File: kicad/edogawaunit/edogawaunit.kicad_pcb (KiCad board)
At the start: 2 copper layers, 26.7 x 22.9 mm, 11 parts, among them J1 Conn_01x03, J2 Conn_01x02, J3 Conn_01x02, SW1 SW_Push, U1 TLP222A-2

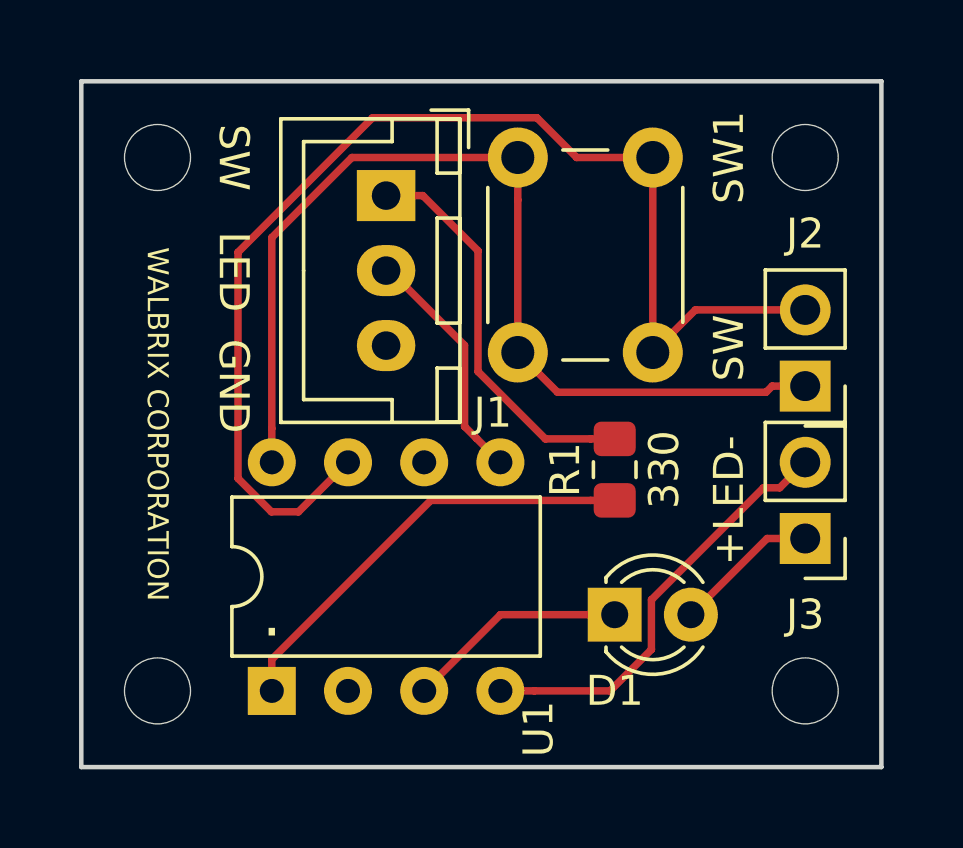
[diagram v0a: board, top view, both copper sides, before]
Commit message: PCBs update
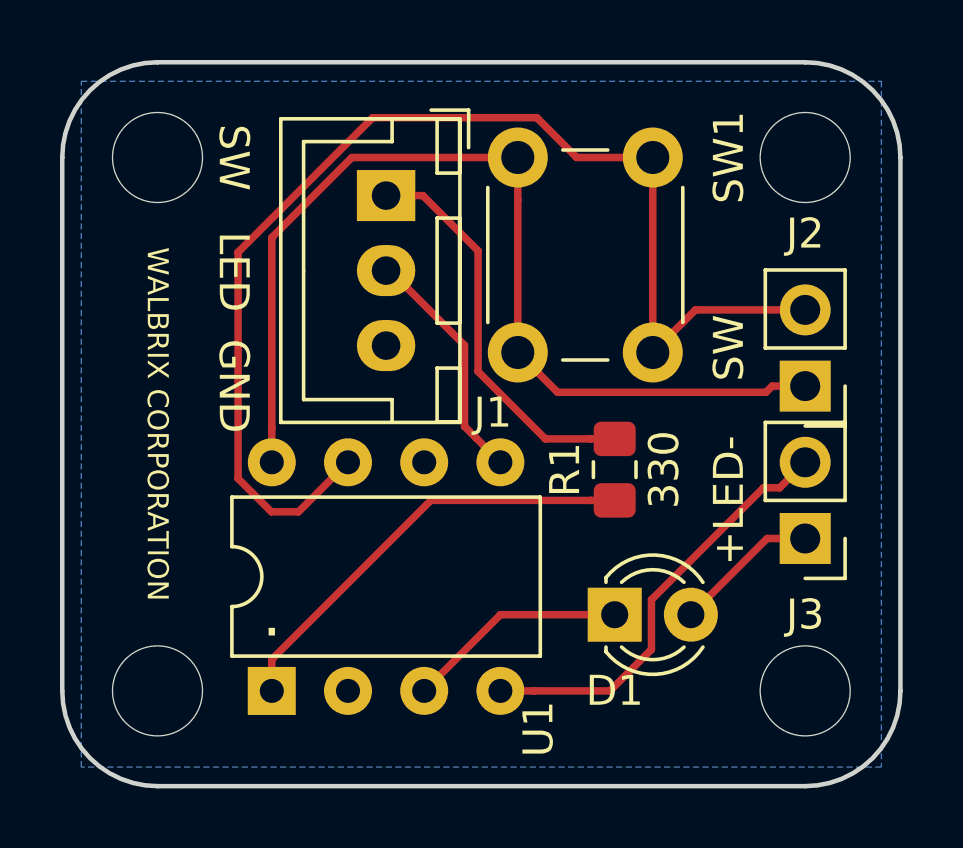
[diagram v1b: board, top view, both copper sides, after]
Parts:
- REF** (x4): value MountingHole_2.2mm_M2 -> MountingHole_3mm; footprint MountingHole:MountingHole_2.2mm_M2 -> MountingHole:MountingHole_3mm
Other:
- board size 26.7 x 22.9 mm -> 27.9 x 24.1 mm
